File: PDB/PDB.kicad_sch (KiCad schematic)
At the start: 0 parts

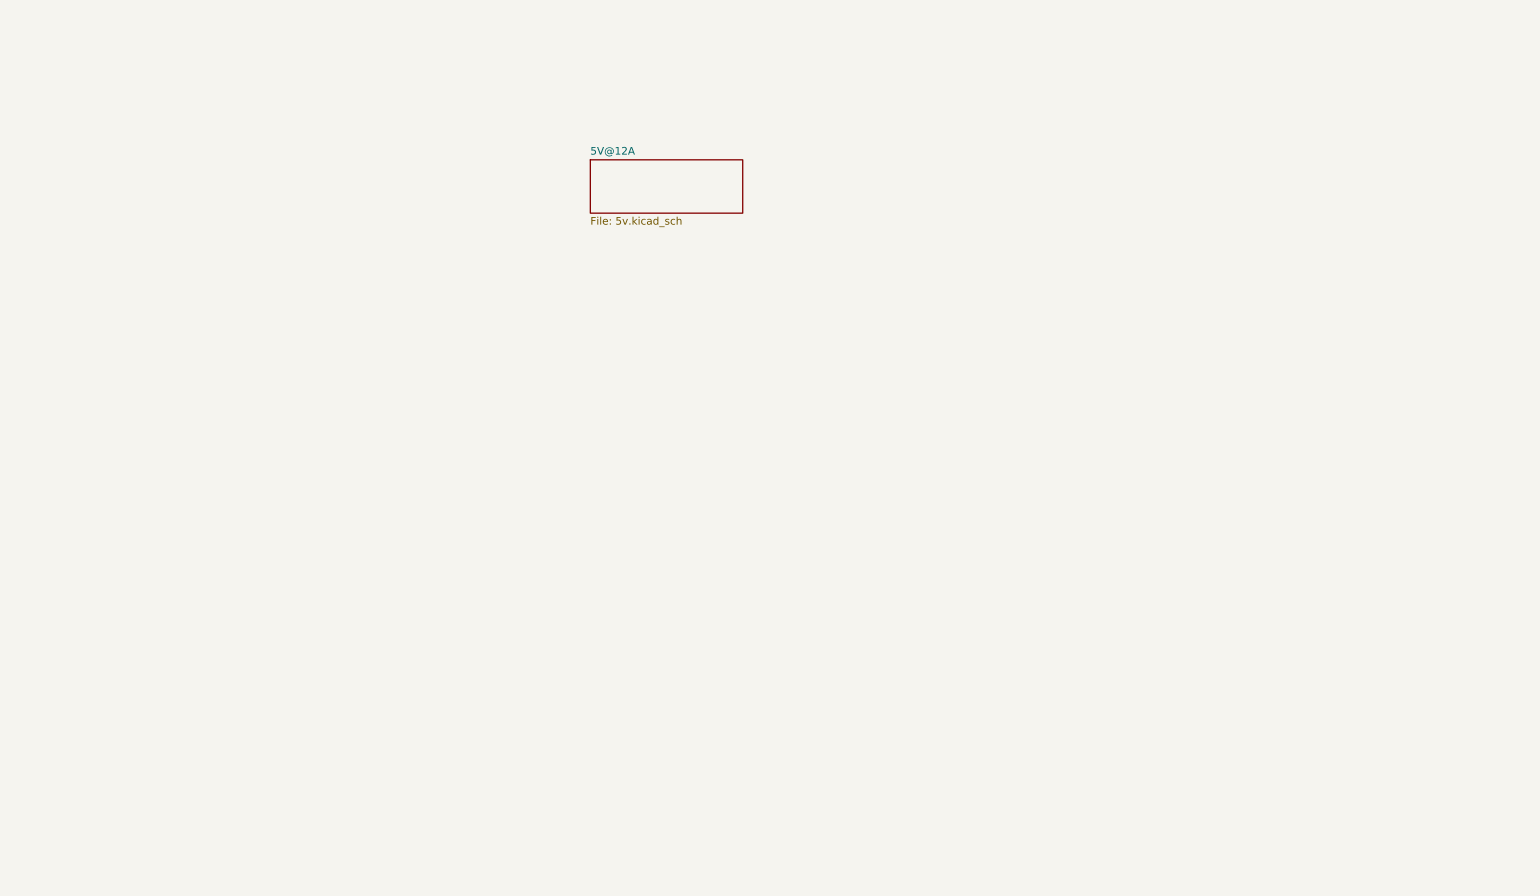
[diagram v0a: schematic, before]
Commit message: did the microcontroller
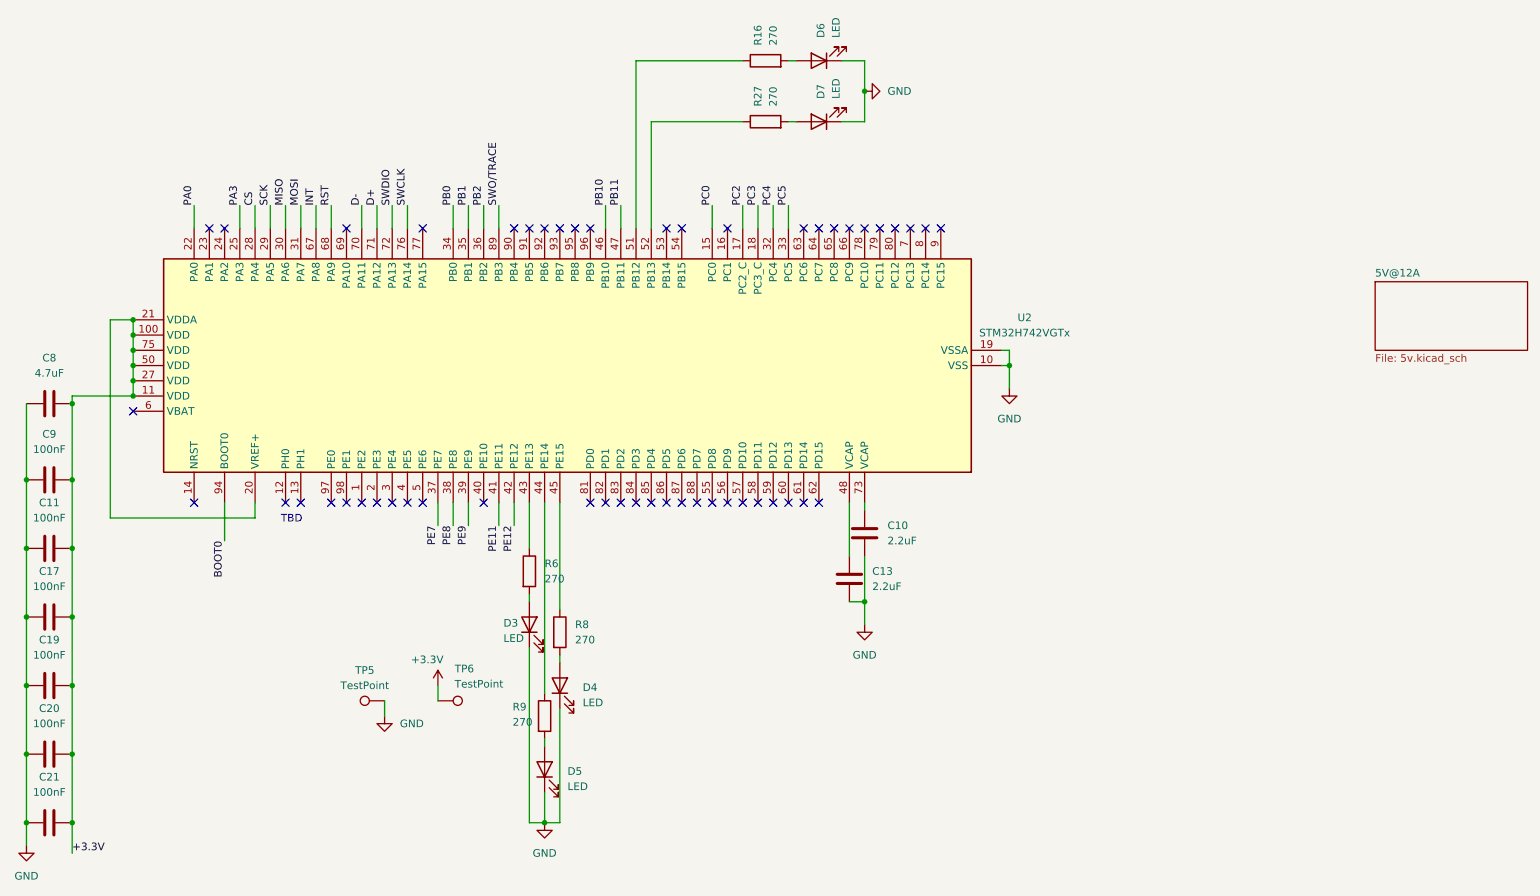
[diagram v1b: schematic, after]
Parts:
- added C10, C13: 2.2uF, Capacitor_SMD:C_1206_3216Metric, symbol Device:C
- added C11, C17, C19, C20, C21, C9: 100nF, Capacitor_SMD:C_1206_3216Metric, symbol Device:C
- added C8: 4.7uF, Capacitor_SMD:C_1206_3216Metric, symbol Device:C
- added D3, D4, D5, D6, D7: LED, LED_SMD:LED_0805_2012Metric, symbol Device:LED
- added R16, R27, R6, R8, R9: 270, Resistor_SMD:R_1206_3216Metric_Pad1.30x1.75mm_HandSolder, symbol Device:R
- added TP5, TP6: TestPoint, TestPoint:TestPoint_Pad_D2.5mm, symbol Connector:TestPoint
- added U2: STM32H742VGTx, Package_QFP:LQFP-100_14x14mm_P0.5mm, symbol MCU_ST_STM32H7:STM32H742VGTx
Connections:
- new net: R27.1, U2.52 (PB13)
- new net: D7.2 (A), R27.2
- new net: C13.2, U2.48 (VCAP)
- new net: R8.1, U2.45 (PE15)
- new net: D4.2 (A), R8.2
- new net: R16.1, U2.51 (PB12)
- new net: D6.2 (A), R16.2
- new net: R9.1, U2.44 (PE14)
- new net: D5.2 (A), R9.2
- new net: R6.1, U2.43 (PE13)
- new net: C10.2, U2.73 (VCAP)
- new net: D3.2 (A), R6.2
- new net +3.3V: C11.2, C17.1, C19.1, C20.1, C21.1, C8.1, C9.1, TP6.1, U2.100 (VDD), U2.11 (VDD), U2.20 (VREF+), U2.21 (VDDA), U2.27 (VDD), U2.50 (VDD), U2.75 (VDD)
- new net BOOT0: U2.94 (BOOT0)
- new net CS: U2.28 (PA4)
- new net D+: U2.71 (PA12)
- new net D-: U2.70 (PA11)
- new net GND: C10.1, C11.1, C13.1, C17.2, C19.2, C20.2, C21.2, C8.2, C9.2, D3.1 (K), D4.1 (K), D5.1 (K), D6.1 (K), D7.1 (K), TP5.1, U2.10 (VSS), U2.19 (VSSA), U2.26 (VSS), U2.49 (VSS), U2.74 (VSS), U2.99 (VSS)
- new net INT: U2.67 (PA8)
- new net MISO: U2.30 (PA6)
- new net MOSI: U2.31 (PA7)
- new net PA0: U2.22 (PA0)
- new net PA3: U2.25 (PA3)
- new net PB0: U2.34 (PB0)
- new net PB1: U2.35 (PB1)
- new net PB10: U2.46 (PB10)
- new net PB11: U2.47 (PB11)
- new net PB2: U2.36 (PB2)
- new net PC0: U2.15 (PC0)
- new net PC2: U2.17 (PC2_C)
- new net PC3: U2.18 (PC3_C)
- new net PC4: U2.32 (PC4)
- new net PC5: U2.33 (PC5)
- new net PE11: U2.41 (PE11)
- new net PE12: U2.42 (PE12)
- new net PE7: U2.37 (PE7)
- new net PE8: U2.38 (PE8)
- new net PE9: U2.39 (PE9)
- new net RST: U2.68 (PA9)
- new net SCK: U2.29 (PA5)
- new net SWCLK: U2.76 (PA14)
- new net SWDIO: U2.72 (PA13)
- new net SWO/TRACE: U2.89 (PB3)
- no-connect marks 0 -> 51
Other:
- note added: "TBD"
